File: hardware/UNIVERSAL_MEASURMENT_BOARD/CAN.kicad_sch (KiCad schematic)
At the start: 17 parts, among them U18 ADM3057EBRWZ

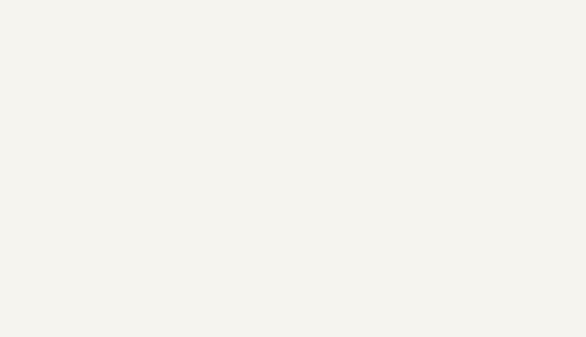
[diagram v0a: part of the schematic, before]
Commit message: clean up project visuals
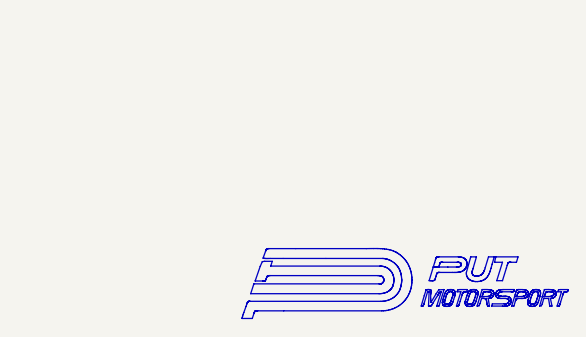
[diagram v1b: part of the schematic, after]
